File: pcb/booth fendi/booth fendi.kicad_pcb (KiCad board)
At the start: 2 copper layers, 144.8 x 99.1 mm, 8 parts, among them J1 Conn_01x01_Female, J2 Conn_01x03_Female, J3 Conn_01x05_Female, J4 Conn_01x03_Female, J5 Conn_01x07_Female, J6 Conn_01x05_Female, J7 Conn_01x03

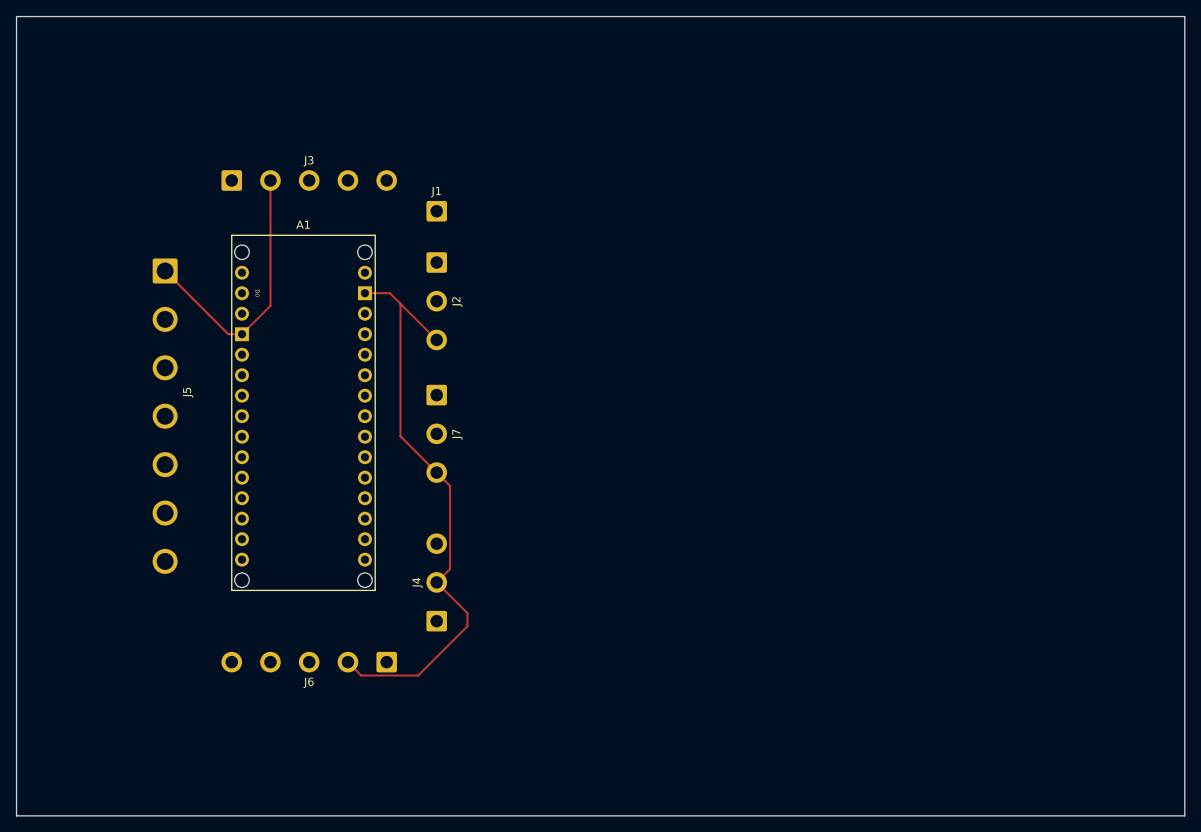
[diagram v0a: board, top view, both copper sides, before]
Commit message: traced no silkscreen
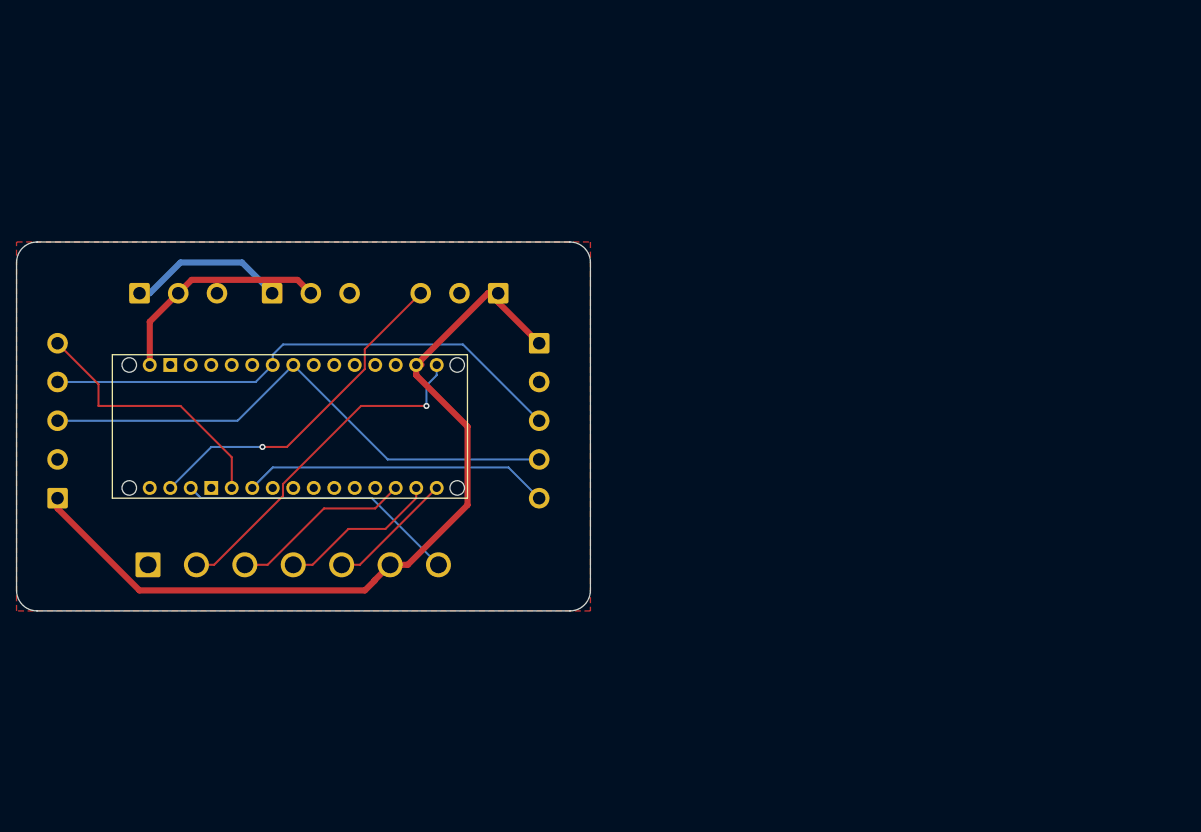
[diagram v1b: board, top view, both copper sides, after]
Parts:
- removed J1: Conn_01x01_Female, Connector_Wire:SolderWire-0.75sqmm_1x01_D1.25mm_OD2.3mm
- moved J3 44.9 mm to (121.9, 97.8), turned to 90 degrees
- moved J6 43.8 mm to (181.6, 78.6), turned to -90 degrees
- moved J4 41.3 mm to (176.5, 72.4), turned to 180 degrees
- moved J2 37.0 mm to (132.1, 72.4), turned to 0 degrees
- moved J5 36.5 mm to (133.1, 106.0), turned to 0 degrees
- moved A1 28.7 mm to (172.7, 88.9), turned to 90 degrees
- moved J7 24.0 mm to (148.5, 72.4), turned to 0 degrees
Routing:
- net GND: track 107.4 -> 0.00 mm
- net +3V3: track 1.12 -> 104.0 mm
- net SDA: track 0.00 -> 67.4 mm
- net SCL: track 0.00 -> 66.3 mm
- net ETH-SCLK: track 0.00 -> 43.1 mm, vias 0 -> 1
- net TTL-DATA: track 0.00 -> 42.5 mm, vias 0 -> 1
- net SB-X: track 0.00 -> 38.2 mm
- net ETH-RST: track 0.00 -> 34.6 mm
- net SA-X: track 0.00 -> 32.8 mm
- net +5V: track 0.00 -> 28.2 mm
- net ETH-SCS: track 0.00 -> 22.6 mm
- net ETH-MOSI: track 0.00 -> 19.9 mm
- net +12V: track 0.00 -> 19.6 mm
- net ETH-MISO: track 0.00 -> 15.7 mm
- added copper zone on F.Cu, net GND
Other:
- board size 144.8 x 99.1 mm -> 71.1 x 45.7 mm

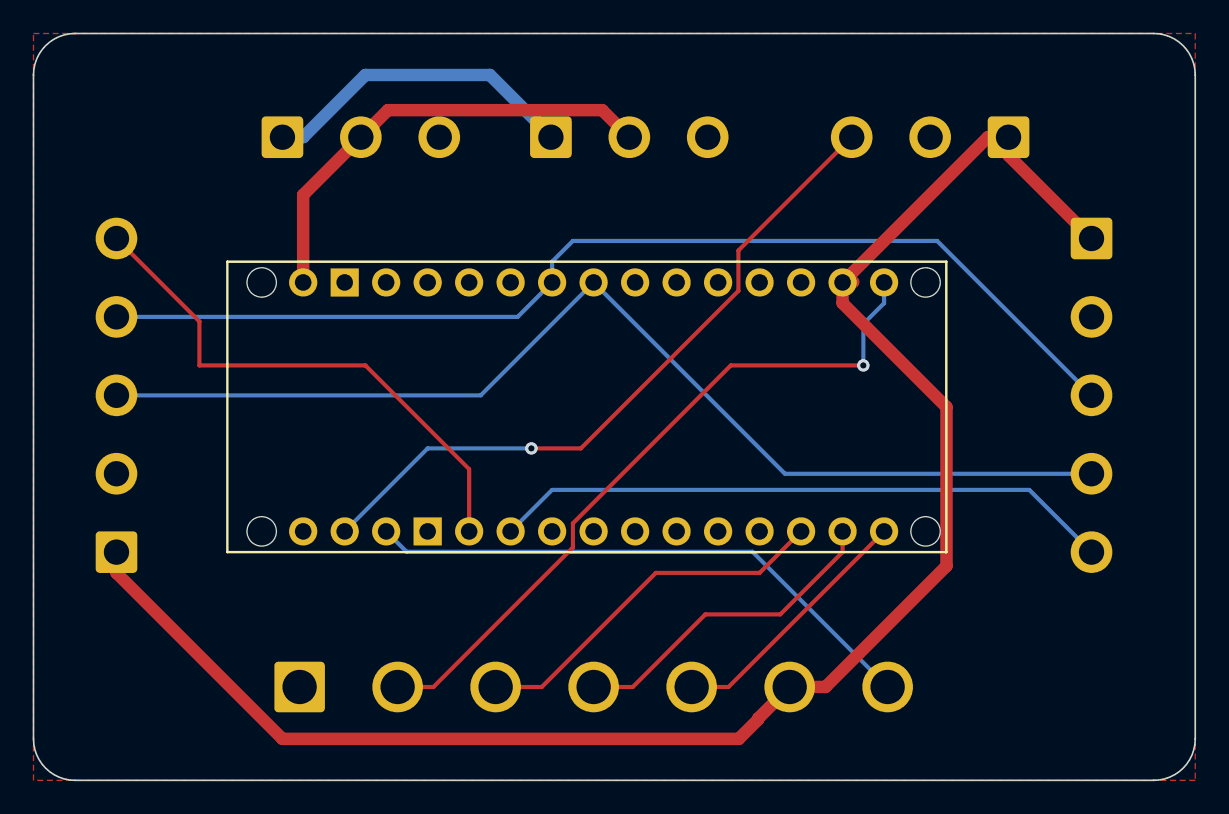
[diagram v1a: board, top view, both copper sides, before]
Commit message: Retraced, need the silkscreen
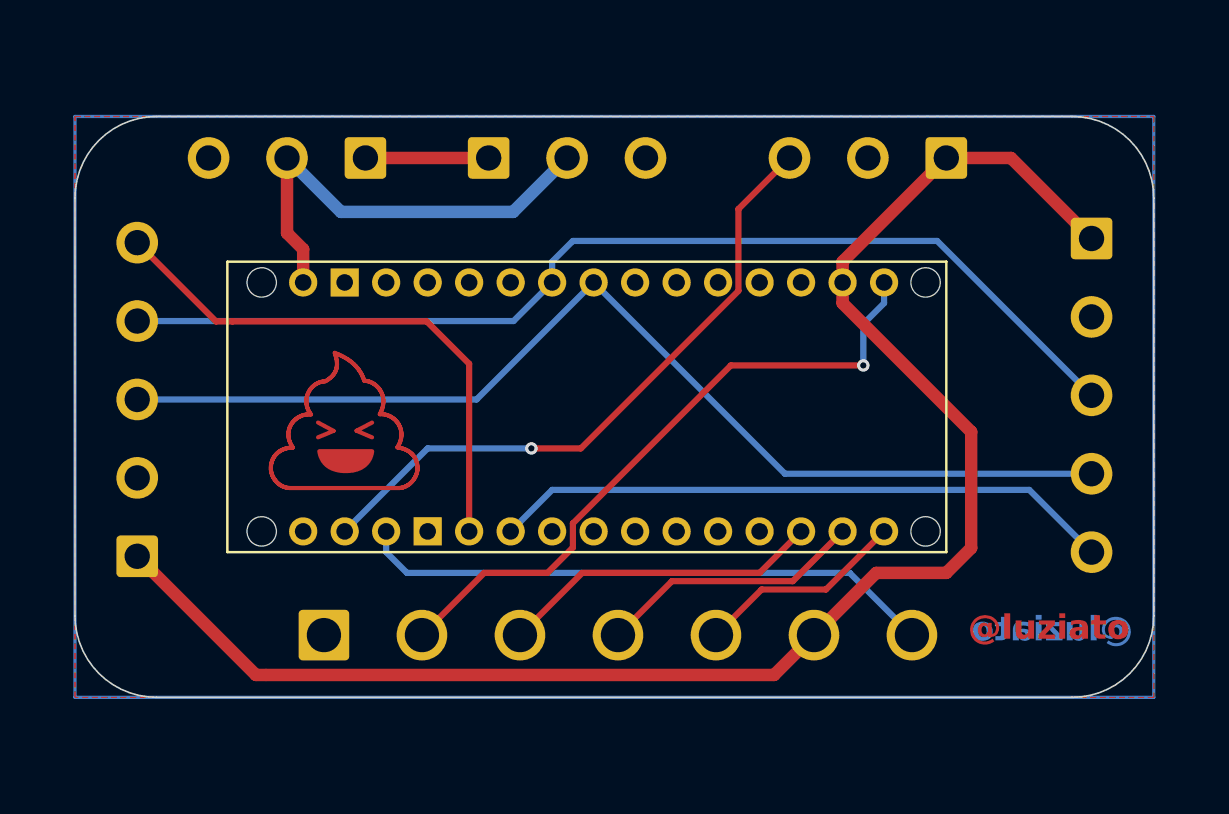
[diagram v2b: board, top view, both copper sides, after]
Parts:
- moved J2 5.24 mm to (137.2, 73.7), turned to 180 degrees
- moved J4 4.02 mm to (172.7, 73.7)
- moved J7 4.02 mm to (144.7, 73.7)
- moved J5 3.51 mm to (134.6, 102.9)
- moved J3 1.30 mm to (123.2, 98.0)
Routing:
- net +12V: track 19.6 -> 7.55 mm
- net +3V3: track 104.0 -> 98.0 mm
- net ETH-MOSI: track 19.9 -> 16.4 mm
- net TTL-DATA: track 42.5 -> 39.6 mm
- net ETH-SCS: track 22.6 -> 19.8 mm
- net ETH-SCLK: track 43.1 -> 40.3 mm
- net ETH-MISO: track 15.7 -> 12.9 mm
- net SDA: track 67.4 -> 66.2 mm
- net SCL: track 66.3 -> 65.1 mm
- net ETH-RST: track 34.6 -> 35.6 mm
- net SA-X: track 32.8 -> 33.7 mm
- added copper zone on B.Cu, net GND
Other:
- board size 71.1 x 45.7 mm -> 66 x 35.6 mm
- board text added: "@luziato"
